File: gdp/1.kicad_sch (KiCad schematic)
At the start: 21 parts, among them IC11 7406, IC3 LM393, IC8 74LS245

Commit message: Placing footprints...
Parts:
- R10, R11, R12, R13, R14, R15, R21, R8, R9: footprint Resistor_THT:R_Axial_DIN0207_L6.3mm_D2.5mm_P7.62mm_Horizontal -> Resistor_THT:R_Axial_DIN0207_L6.3mm_D2.5mm_P10.16mm_Horizontal
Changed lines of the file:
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@@
 			)
 		)
-		(property "Footprint" "Resistor_THT:R_Axial_DIN0207_L6.3mm_D2.5mm_P7.62mm_Horizontal"
+		(property "Footprint" "Resistor_THT:R_Axial_DIN0207_L6.3mm_D2.5mm_P10.16mm_Horizontal"
 			(at 202.692 110.49 90)
 			(effects
@@
 			)
 		)
-		(property "Footprint" "Resistor_THT:R_Axial_DIN0207_L6.3mm_D2.5mm_P7.62mm_Horizontal"
+		(property "Footprint" "Resistor_THT:R_Axial_DIN0207_L6.3mm_D2.5mm_P10.16mm_Horizontal"
 			(at 187.452 110.49 90)
 			(effects
@@
 			)
 		)
-		(property "Footprint" "Resistor_THT:R_Axial_DIN0207_L6.3mm_D2.5mm_P7.62mm_Horizontal"
+		(property "Footprint" "Resistor_THT:R_Axial_DIN0207_L6.3mm_D2.5mm_P10.16mm_Horizontal"
 			(at 174.752 110.49 90)
 			(effects
@@
 			)
 		)
-		(property "Footprint" "Resistor_THT:R_Axial_DIN0207_L6.3mm_D2.5mm_P7.62mm_Horizontal"
+		(property "Footprint" "Resistor_THT:R_Axial_DIN0207_L6.3mm_D2.5mm_P10.16mm_Horizontal"
 			(at 219.71 109.093 90)
 			(effects
@@
 			)
 		)
-		(property "Footprint" "Resistor_THT:R_Axial_DIN0207_L6.3mm_D2.5mm_P7.62mm_Horizontal"
+		(property "Footprint" "Resistor_THT:R_Axial_DIN0207_L6.3mm_D2.5mm_P10.16mm_Horizontal"
 			(at 219.71 121.793 90)
 			(effects
@@
 			)
 		)
-		(property "Footprint" "Resistor_THT:R_Axial_DIN0207_L6.3mm_D2.5mm_P7.62mm_Horizontal"
+		(property "Footprint" "Resistor_THT:R_Axial_DIN0207_L6.3mm_D2.5mm_P10.16mm_Horizontal"
 			(at 195.072 110.49 90)
 			(effects
@@
 			)
 		)
-		(property "Footprint" "Resistor_THT:R_Axial_DIN0207_L6.3mm_D2.5mm_P7.62mm_Horizontal"
+		(property "Footprint" "Resistor_THT:R_Axial_DIN0207_L6.3mm_D2.5mm_P10.16mm_Horizontal"
 			(at 219.71 115.443 90)
 			(effects
@@
 			)
 		)
-		(property "Footprint" "Resistor_THT:R_Axial_DIN0207_L6.3mm_D2.5mm_P7.62mm_Horizontal"
+		(property "Footprint" "Resistor_THT:R_Axial_DIN0207_L6.3mm_D2.5mm_P10.16mm_Horizontal"
 			(at 219.71 128.143 90)
 			(effects
@@
 			)
 		)
-		(property "Footprint" "Resistor_THT:R_Axial_DIN0207_L6.3mm_D2.5mm_P7.62mm_Horizontal"
+		(property "Footprint" "Resistor_THT:R_Axial_DIN0207_L6.3mm_D2.5mm_P10.16mm_Horizontal"
 			(at 159.512 120.015 90)
 			(effects

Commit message: Maps footprints PCB -> sch
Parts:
- CK23: footprint Capacitor_THT:C_Disc_D4.3mm_W1.9mm_P5.00mm -> Capacitor_THT:CP_Radial_Tantal_D6.0mm_P5.00mm
- R10, R15, R21, R8, R9: footprint Resistor_THT:R_Axial_DIN0207_L6.3mm_D2.5mm_P10.16mm_Horizontal -> GDP:R_XL
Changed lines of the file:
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@@
 			)
 		)
-		(property "Footprint" "Capacitor_THT:C_Disc_D4.3mm_W1.9mm_P5.00mm"
+		(property "Footprint" "Capacitor_THT:CP_Radial_Tantal_D6.0mm_P5.00mm"
 			(at 224.79 58.42 0)
 			(effects
@@
 			)
 		)
-		(property "Footprint" "Resistor_THT:R_Axial_DIN0207_L6.3mm_D2.5mm_P10.16mm_Horizontal"
+		(property "Footprint" "GDP:R_XL"
 			(at 174.752 110.49 90)
 			(effects
@@
 			)
 		)
-		(property "Footprint" "Resistor_THT:R_Axial_DIN0207_L6.3mm_D2.5mm_P10.16mm_Horizontal"
+		(property "Footprint" "GDP:R_XL"
 			(at 219.71 109.093 90)
 			(effects
@@
 			)
 		)
-		(property "Footprint" "Resistor_THT:R_Axial_DIN0207_L6.3mm_D2.5mm_P10.16mm_Horizontal"
+		(property "Footprint" "GDP:R_XL"
 			(at 219.71 121.793 90)
 			(effects
@@
 			)
 		)
-		(property "Footprint" "Resistor_THT:R_Axial_DIN0207_L6.3mm_D2.5mm_P10.16mm_Horizontal"
+		(property "Footprint" "GDP:R_XL"
 			(at 219.71 115.443 90)
 			(effects
@@
 			)
 		)
-		(property "Footprint" "Resistor_THT:R_Axial_DIN0207_L6.3mm_D2.5mm_P10.16mm_Horizontal"
+		(property "Footprint" "GDP:R_XL"
 			(at 219.71 128.143 90)
 			(effects

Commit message: Fixes footprint references in sch
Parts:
- R11, R12, R13, R14: footprint Resistor_THT:R_Axial_DIN0207_L6.3mm_D2.5mm_P10.16mm_Horizontal -> GDP:R_XL
- ST1: footprint Connector_PinHeader_2.54mm:PinHeader_1x06_P2.54mm_Vertical -> GDP:PWR
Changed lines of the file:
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@@
 			)
 		)
-		(property "Footprint" "Resistor_THT:R_Axial_DIN0207_L6.3mm_D2.5mm_P10.16mm_Horizontal"
+		(property "Footprint" "GDP:R_XL"
 			(at 202.692 110.49 90)
 			(effects
@@
 			)
 		)
-		(property "Footprint" "Resistor_THT:R_Axial_DIN0207_L6.3mm_D2.5mm_P10.16mm_Horizontal"
+		(property "Footprint" "GDP:R_XL"
 			(at 187.452 110.49 90)
 			(effects
@@
 			)
 		)
-		(property "Footprint" "Resistor_THT:R_Axial_DIN0207_L6.3mm_D2.5mm_P10.16mm_Horizontal"
+		(property "Footprint" "GDP:R_XL"
 			(at 195.072 110.49 90)
 			(effects
@@
 			)
 		)
-		(property "Footprint" "Connector_PinHeader_2.54mm:PinHeader_1x06_P2.54mm_Vertical"
+		(property "Footprint" "GDP:PWR"
 			(at 243.84 61.595 0)
 			(effects
@@
 			)
 		)
-		(property "Footprint" "Resistor_THT:R_Axial_DIN0207_L6.3mm_D2.5mm_P10.16mm_Horizontal"
+		(property "Footprint" "GDP:R_XL"
 			(at 159.512 120.015 90)
 			(effects

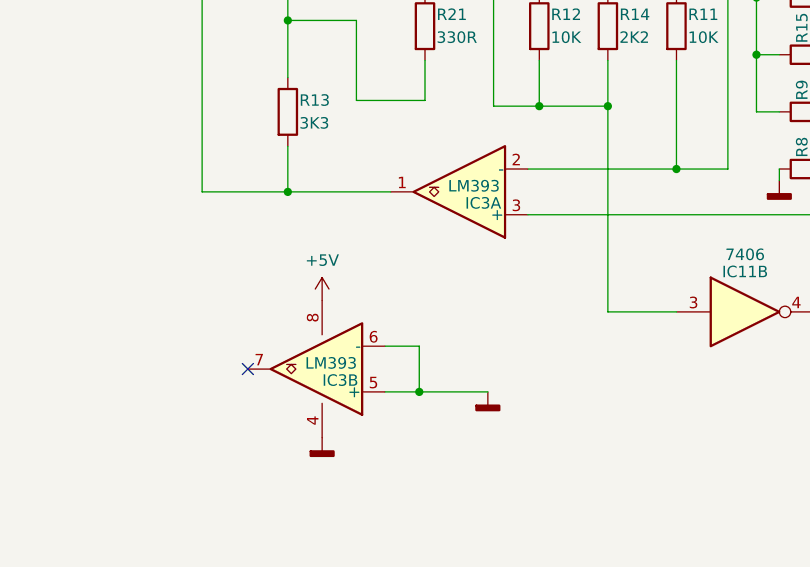
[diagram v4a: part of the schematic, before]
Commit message: Fixes GND issue (R32)
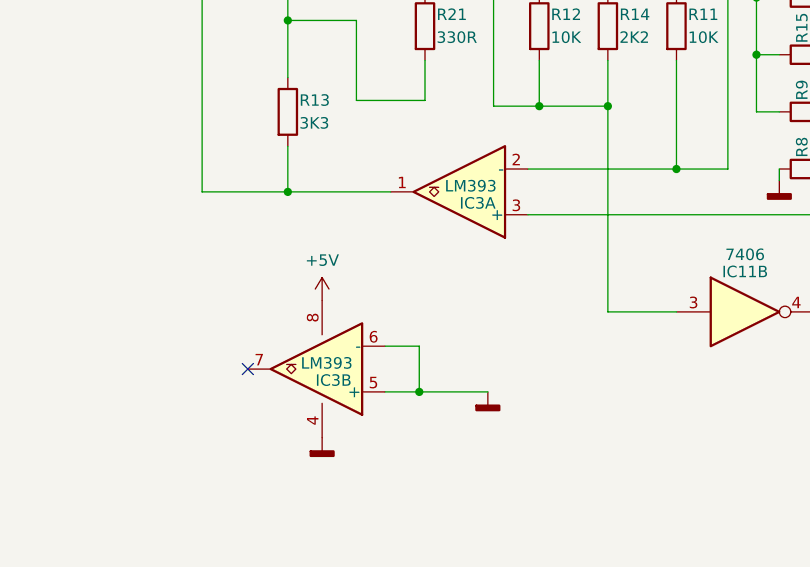
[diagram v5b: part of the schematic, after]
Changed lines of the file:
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@@
 		(dnp no)
 		(property "Reference" "IC3"
-			(at 180.975 130.175 0)
-			(effects
-				(font
-					(size 1.27 1.27)
-				)
-				(justify right)
+			(at 182.372 130.175 0)
+			(do_not_autoplace yes)
+			(effects
+				(font
+					(size 1.27 1.27)
+				)
 			)
 		)
 		(property "Value" "LM393"
-			(at 179.07 128.27 0)
-			(effects
-				(font
-					(size 1.27 1.27)
-				)
-				(justify right)
+			(at 181.61 128.27 0)
+			(do_not_autoplace yes)
+			(effects
+				(font
+					(size 1.27 1.27)
+				)
 			)
 		)
@@
 		(dnp no)
 		(property "Reference" "IC3"
-			(at 165.1 149.86 0)
-			(effects
-				(font
-					(size 1.27 1.27)
-				)
-				(justify right)
+			(at 166.37 149.86 0)
+			(do_not_autoplace yes)
+			(effects
+				(font
+					(size 1.27 1.27)
+				)
 			)
 		)
 		(property "Value" "LM393"
-			(at 163.195 147.955 0)
-			(effects
-				(font
-					(size 1.27 1.27)
-				)
-				(justify right)
-			)
-		)
+			(at 165.608 147.955 0)
+			(do_not_autoplace yes)
+			(effects
+				(font
+					(size 1.27 1.27)
+				)
+			)
+		)
